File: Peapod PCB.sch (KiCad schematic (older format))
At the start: 17 parts, among them J1 CONN_01X01, J2 CONN_01X02, J3 CONN_01X01, J4 CONN_01X01, J5 CONN_01X01, J6 CONN_01X01, J7 CONN_01X02, U1 ESP8266

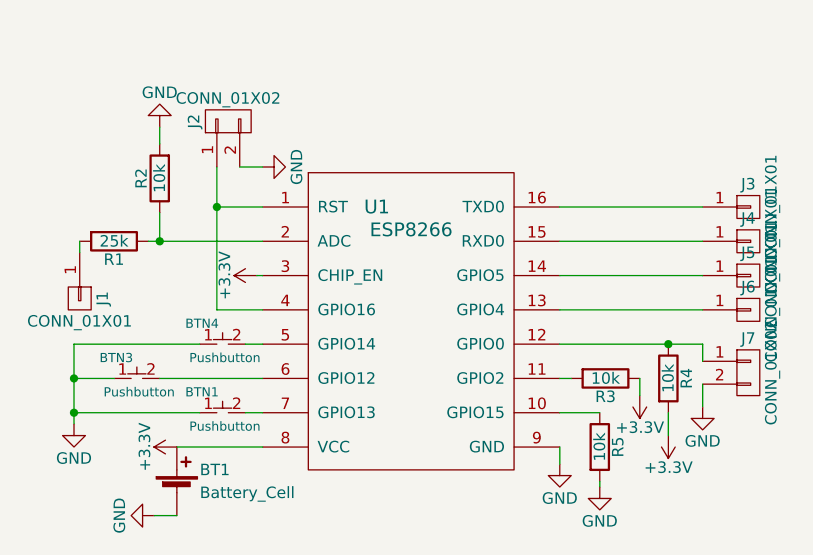
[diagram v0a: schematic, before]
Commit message: Updated schematic
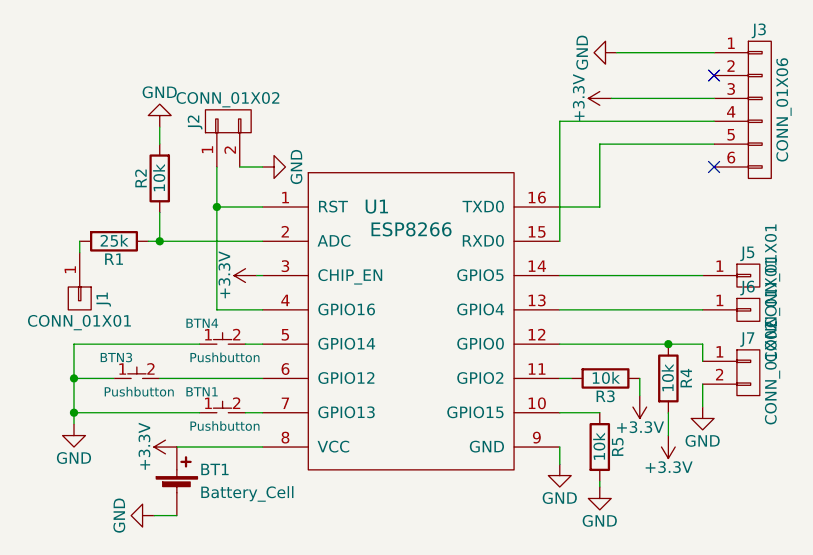
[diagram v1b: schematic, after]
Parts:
- removed J3, J4: CONN_01X01, mod:Alligator Pad, symbol CONN_01X01
- added J3: CONN_01X06, Pin_Headers:Pin_Header_Straight_1x06_Pitch2.54mm, symbol CONN_01X06
- R3, R5: footprint (none) -> Resistors_SMD:R_0805_HandSoldering
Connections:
- net +3V3: now also J3.3 (P3)
- net GND: now also J3.1 (P1)
- net at U1.15 (RXD0): now also J3.4 (P4)
- net at U1.16 (TXD0): now also J3.5 (P5)
- no-connect marks 0 -> 2
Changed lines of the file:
@@
 $EndComp
 $Comp
-L GND #PWR5
+L GND #PWR01
 U 1 1 59932223
 P 4850 4225
-F 0 "#PWR5" H 4850 3975 50  0001 C CNN
+F 0 "#PWR01" H 4850 3975 50  0001 C CNN
 F 1 "GND" H 4850 4075 50  0000 C CNN
 F 2 "" H 4850 4225 50  0001 C CNN
@@
 $EndComp
 $Comp
-L GND #PWR6
+L GND #PWR02
 U 1 1 59932907
 P 6800 4100
-F 0 "#PWR6" H 6800 3850 50  0001 C CNN
+F 0 "#PWR02" H 6800 3850 50  0001 C CNN
 F 1 "GND" H 6800 3950 50  0000 C CNN
 F 2 "" H 6800 4100 50  0001 C CNN
@@
 $EndComp
 $Comp
-L GND #PWR1
+L GND #PWR03
 U 1 1 5993357D
 P 4500 3825
-F 0 "#PWR1" H 4500 3575 50  0001 C CNN
+F 0 "#PWR03" H 4500 3575 50  0001 C CNN
 F 1 "GND" H 4500 3675 50  0000 C CNN
 F 2 "" H 4500 3825 50  0001 C CNN
 F 3 "" H 4500 3825 50  0001 C CNN
 	1    4500 3825
-	1    0    0    -1
-$EndComp
-$Comp
-L CONN_01X01 J3
-U 1 1 59933B2D
-P 7450 2875
-F 0 "J3" H 7450 2975 50  0000 C CNN
-F 1 "CONN_01X01" V 7550 2875 50  0000 C CNN
-F 2 "mod:Alligator Pad" H 7450 2875 50  0001 C CNN
-F 3 "" H 7450 2875 50  0001 C CNN
-	1    7450 2875
-	1    0    0    -1
-$EndComp
-$Comp
-L CONN_01X01 J4
-U 1 1 59933BB9
-P 7450 3025
-F 0 "J4" H 7450 3125 50  0000 C CNN
-F 1 "CONN_01X01" V 7550 3025 50  0000 C CNN
-F 2 "mod:Alligator Pad" H 7450 3025 50  0001 C CNN
-F 3 "" H 7450 3025 50  0001 C CNN
-	1    7450 3025
 	1    0    0    -1
 $EndComp
@@
 $EndComp
 $Comp
-L +3.3V #PWR2
+L +3.3V #PWR04
 U 1 1 59933FE4
 P 5300 3175
-F 0 "#PWR2" H 5300 3025 50  0001 C CNN
+F 0 "#PWR04" H 5300 3025 50  0001 C CNN
 F 1 "+3.3V" H 5300 3315 50  0000 C CNN
 F 2 "" H 5300 3175 50  0001 C CNN
@@
 $EndComp
 $Comp
-L +3.3V #PWR4
+L +3.3V #PWR05
 U 1 1 59934256
 P 4950 3925
-F 0 "#PWR4" H 4950 3775 50  0001 C CNN
+F 0 "#PWR05" H 4950 3775 50  0001 C CNN
 F 1 "+3.3V" H 4950 4065 50  0000 C CNN
 F 2 "" H 4950 3925 50  0001 C CNN
@@
 	4500 3775 5050 3775
 Wire Wire Line
-	4500 3475 4500 3625
-Wire Wire Line
-	4500 3625 4500 3775
-Wire Wire Line
-	4500 3775 4500 3825
+	4500 3475 4500 3825
 Connection ~ 4500 3625
 Wire Wire Line
@@
 Wire Wire Line
 	6625 3325 7250 3325
-Wire Wire Line
-	6625 2875 7250 2875
-Wire Wire Line
-	6625 3025 7250 3025
 Wire Wire Line
 	4500 3475 5050 3475
@@
 	4950 4225 4850 4225
 Wire Wire Line
-	5125 2700 5125 2875
-Wire Wire Line
-	5125 2875 5125 3325
+	5125 2700 5125 3325
 Wire Wire Line
 	5125 2875 5325 2875
 Connection ~ 5125 2875
 Wire Wire Line
-	4825 3025 4875 3025
-Wire Wire Line
-	4875 3025 5325 3025
+	4825 3025 5325 3025
 $Comp
 L R R2
@@
 $EndComp
 Wire Wire Line
-	6625 3475 7100 3475
-Wire Wire Line
-	7100 3475 7250 3475
+	6625 3475 7250 3475
 Connection ~ 7100 3475
 $Comp
@@
 $EndComp
 $Comp
-L GND #PWR3
+L GND #PWR06
 U 1 1 599363AF
 P 5325 2700
-F 0 "#PWR3" H 5325 2450 50  0001 C CNN
+F 0 "#PWR06" H 5325 2450 50  0001 C CNN
 F 1 "GND" H 5325 2550 50  0000 C CNN
 F 2 "" H 5325 2700 50  0001 C CNN
@@
 $EndComp
 $Comp
-L +3.3V #PWR7
+L +3.3V #PWR07
 U 1 1 599466C8
 P 7100 3875
-F 0 "#PWR7" H 7100 3725 50  0001 C CNN
+F 0 "#PWR07" H 7100 3725 50  0001 C CNN
 F 1 "+3.3V" H 7100 4015 50  0000 C CNN
 F 2 "" H 7100 3875 50  0001 C CNN
@@
 F 0 "R3" V 6905 3625 50  0000 C CNN
 F 1 "10k" V 6825 3625 50  0000 C CNN
-F 2 "" V 6755 3625 50  0001 C CNN
+F 2 "Resistors_SMD:R_0805_HandSoldering" V 6755 3625 50  0001 C CNN
 F 3 "" H 6825 3625 50  0001 C CNN
 	1    6825 3625
@@
 F 0 "R5" V 6880 3925 50  0000 C CNN
 F 1 "10k" V 6800 3925 50  0000 C CNN
-F 2 "" V 6730 3925 50  0001 C CNN
+F 2 "Resistors_SMD:R_0805_HandSoldering" V 6730 3925 50  0001 C CNN
 F 3 "" H 6800 3925 50  0001 C CNN
 	1    6800 3925
@@
 	6625 3775 6800 3775
 $Comp
-L +3.3V #PWR?
+L +3.3V #PWR08
 U 1 1 59948486
 P 6975 3700
-F 0 "#PWR?" H 6975 3550 50  0001 C CNN
+F 0 "#PWR08" H 6975 3550 50  0001 C CNN
 F 1 "+3.3V" H 6975 3840 50  0000 C CNN
 F 2 "" H 6975 3700 50  0001 C CNN
@@
 	4875 2900 4875 3025
 $Comp
-L GND #PWR?
+L GND #PWR09
 U 1 1 5994872F
 P 4875 2525
-F 0 "#PWR?" H 4875 2275 50  0001 C CNN
+F 0 "#PWR09" H 4875 2275 50  0001 C CNN
 F 1 "GND" H 4875 2375 50  0000 C CNN
 F 2 "" H 4875 2525 50  0001 C CNN
@@
 	4875 2525 4875 2600
 $Comp
-L GND #PWR?
+L GND #PWR010
 U 1 1 599488CC
 P 7250 3750
-F 0 "#PWR?" H 7250 3500 50  0001 C CNN
+F 0 "#PWR010" H 7250 3500 50  0001 C CNN
 F 1 "GND" H 7250 3600 50  0000 C CNN
 F 2 "" H 7250 3750 50  0001 C CNN
@@
 $EndComp
 $Comp
-L GND #PWR?
+L GND #PWR011
 U 1 1 59948924
 P 6625 4000
-F 0 "#PWR?" H 6625 3750 50  0001 C CNN
+F 0 "#PWR011" H 6625 3750 50  0001 C CNN
 F 1 "GND" H 6625 3850 50  0000 C CNN
 F 2 "" H 6625 4000 50  0001 C CNN
@@
 Wire Wire Line
 	5325 3925 4950 3925
+$Comp
+L CONN_01X06 J3
+U 1 1 59947FD8
+P 7500 2450
+F 0 "J3" H 7500 2800 50  0000 C CNN
+F 1 "CONN_01X06" V 7600 2450 50  0000 C CNN
+F 2 "Pin_Headers:Pin_Header_Straight_1x06_Pitch2.54mm" H 7500 2450 50  0001 C CNN
+F 3 "" H 7500 2450 50  0001 C CNN
+	1    7500 2450
+	1    0    0    -1
+$EndComp
+$Comp
+L GND #PWR012
+U 1 1 599480D5
+P 6875 2200
+F 0 "#PWR012" H 6875 1950 50  0001 C CNN
+F 1 "GND" H 6875 2050 50  0000 C CNN
+F 2 "" H 6875 2200 50  0001 C CNN
+F 3 "" H 6875 2200 50  0001 C CNN
+	1    6875 2200
+	0    1    1    0
+$EndComp
+Wire Wire Line
+	6875 2200 7300 2200
+$Comp
+L +3.3V #PWR013
+U 1 1 599481A2
+P 6850 2400
+F 0 "#PWR013" H 6850 2250 50  0001 C CNN
+F 1 "+3.3V" H 6850 2540 50  0000 C CNN
+F 2 "" H 6850 2400 50  0001 C CNN
+F 3 "" H 6850 2400 50  0001 C CNN
+	1    6850 2400
+	0    -1   -1   0
+$EndComp
+Wire Wire Line
+	6850 2400 7300 2400
+Wire Wire Line
+	6625 2875 6800 2875
+Wire Wire Line
+	6800 2875 6800 2600
+Wire Wire Line
+	6800 2600 7300 2600
+Wire Wire Line
+	6625 3025 6625 2500
+Wire Wire Line
+	6625 2500 7300 2500
+NoConn ~ 7300 2700
+NoConn ~ 7300 2300
 $EndSCHEMATC
